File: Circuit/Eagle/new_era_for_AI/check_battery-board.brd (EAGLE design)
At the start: 94 x 70 mm, 32 parts

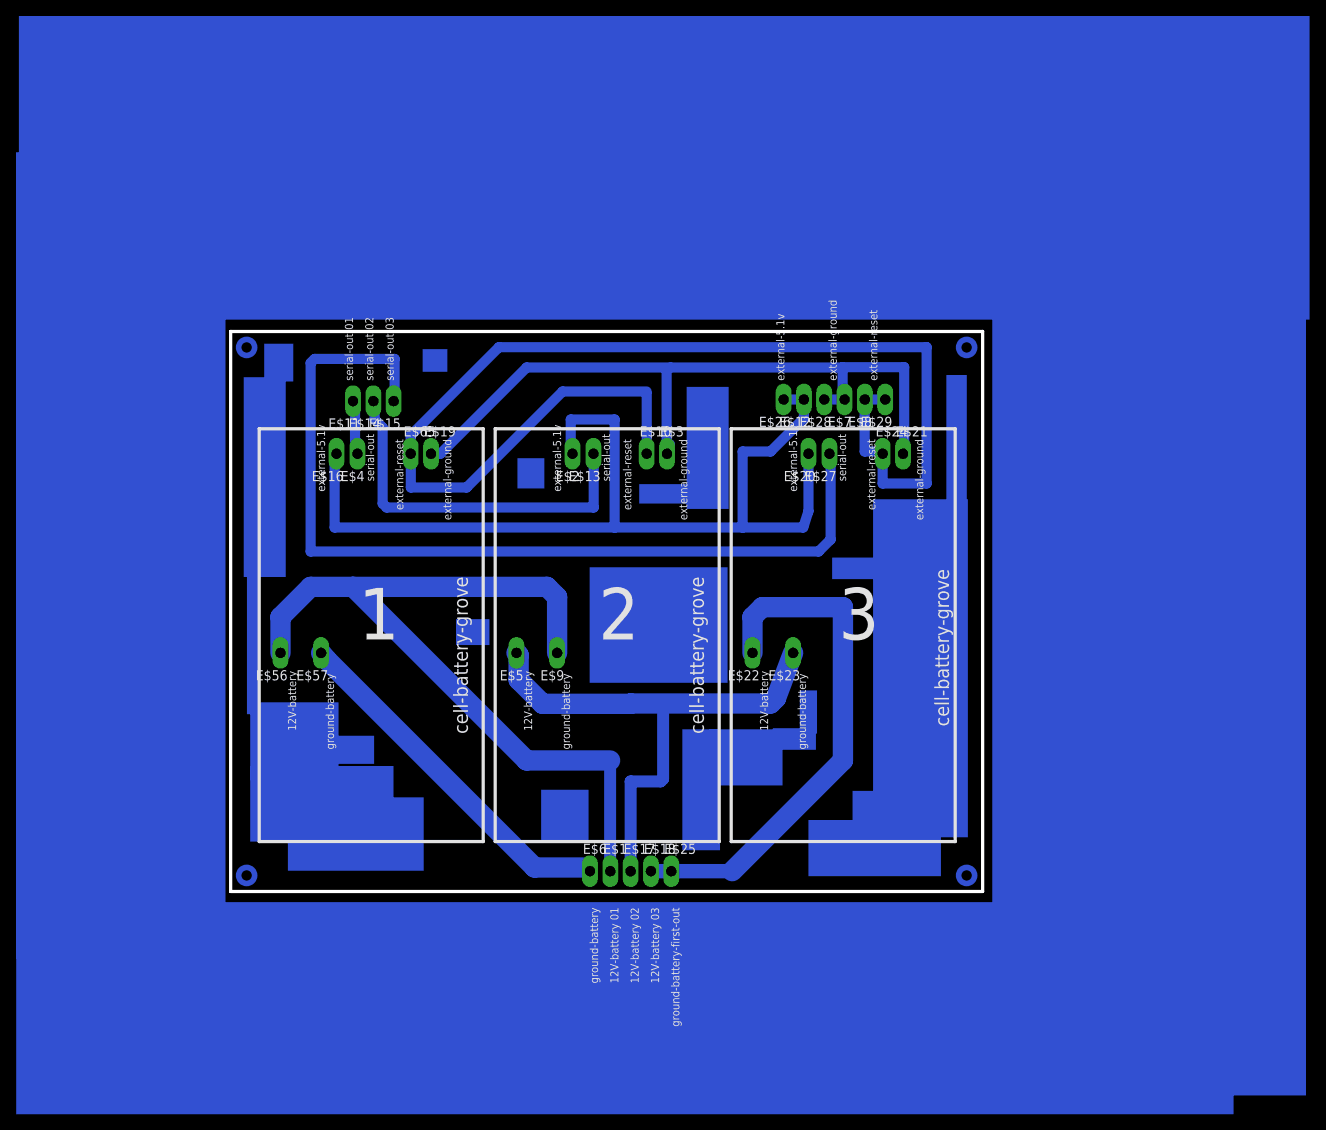
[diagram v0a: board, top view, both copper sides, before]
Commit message: .
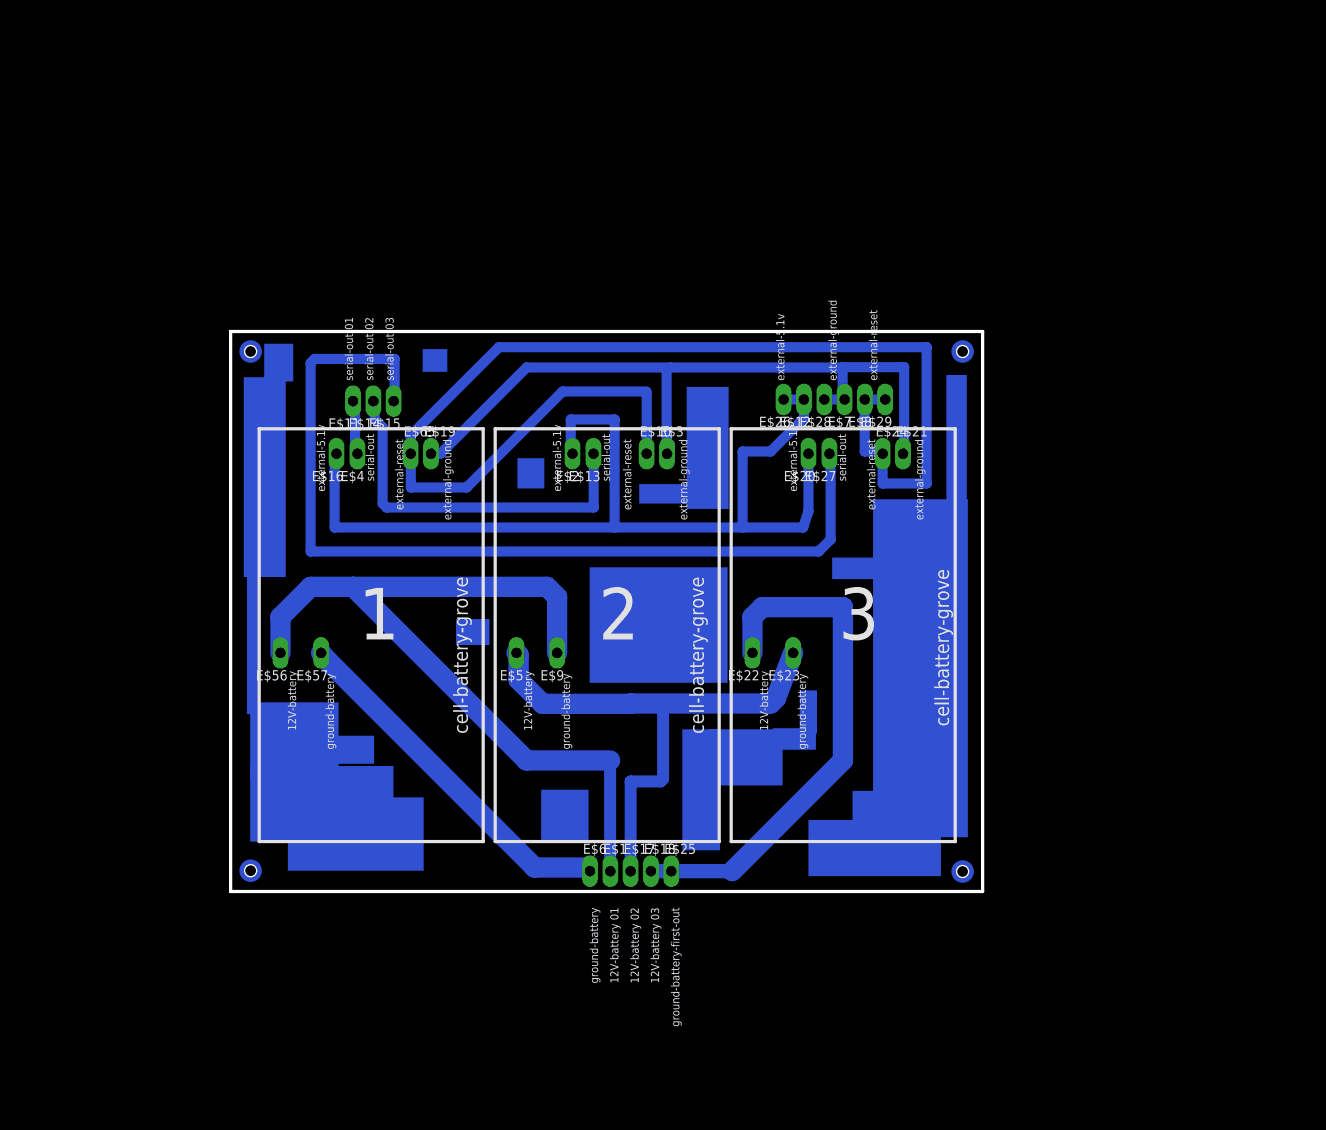
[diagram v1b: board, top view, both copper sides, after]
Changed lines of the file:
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@@
 <setting verticaltext="up"/>
 </settings>
-<grid distance="0.003125" unitdist="mic" unit="mm" style="lines" multiple="1" display="yes" altdistance="0.003125" altunitdist="mic" altunit="mm"/>
+<grid distance="0.5" unitdist="mm" unit="mm" style="lines" multiple="1" display="yes" altdistance="0.003125" altunitdist="mic" altunit="mm"/>
 <layers>
-<layer number="1" name="Top" color="4" fill="1" visible="no" active="yes"/>
+<layer number="1" name="Top" color="4" fill="1" visible="yes" active="yes"/>
 <layer number="2" name="Route2" color="1" fill="3" visible="no" active="no"/>
 <layer number="3" name="Route3" color="4" fill="3" visible="no" active="no"/>
@@
 <layer number="45" name="Holes" color="7" fill="1" visible="yes" active="yes"/>
 <layer number="46" name="Milling" color="3" fill="1" visible="no" active="yes"/>
-<layer number="47" name="Measures" color="7" fill="1" visible="no" active="yes"/>
+<layer number="47" name="Measures" color="7" fill="1" visible="yes" active="yes"/>
 <layer number="48" name="Document" color="7" fill="1" visible="no" active="yes"/>
 <layer number="49" name="Reference" color="7" fill="1" visible="no" active="yes"/>
@@
 </layers>
 <board>
-<fusionsync huburn="a.cGVyc29uYWw6dWUyZDdmOThi" projecturn="a.cGVyc29uYWw6dWUyZDdmOThiIzIwMjAxMTA1MzUwMDc2Njgx" f3durn="urn:adsk.wipprod:dm.lineage:Sfrp7S-jSqKYQXxY8w-WgQ" pcbguid="81441e6f-d9b8-4305-a09b-ce2376f146d5" lastpulledtime="" lastsyncedchangeguid="9a0dcba4-15db-f250-db5e-a71cff48e025" latestrevisionid="" lastsyncedrevisionid="" lastboardhashguid="" lastpushedtime="" linktopcb3d="false"/>
+<fusionsync huburn="a.cGVyc29uYWw6dWUyZDdmOThi" projecturn="a.cGVyc29uYWw6dWUyZDdmOThiIzIwMjAxMTA1MzUwMDc2Njgx" f3durn="urn:adsk.wipprod:dm.lineage:0ixU6gNjSq-owvs7GqFS4g" pcbguid="" lastpulledtime="" lastsyncedchangeguid="9a0dcba4-15db-f250-db5e-a71cff48e025" latestrevisionid="9c5196f6-a430-4b2d-92e1-2361bd45ccda" lastsyncedrevisionid="9c5196f6-a430-4b2d-92e1-2361bd45ccda" lastboardhashguid="3221ca91-becd-a7e8-faa7-446c98a98a6c" lastpushedtime="2024-01-14T22:33:02Z" linktopcb3d="true"/>
 <plain>
 <text x="19.933525" y="53.274865625" size="1.016" layer="21" rot="R90">serial-out</text>
@@
 <text x="48" y="33.5" size="6.4516" layer="21">2</text>
 <text x="78" y="33.5" size="6.4516" layer="21">3</text>
-<wire x1="2" y1="72" x2="96" y2="72" width="0.4064" layer="20"/>
-<wire x1="96" y1="2" x2="2" y2="2" width="0.4064" layer="20"/>
 <dimension x1="2" y1="72" x2="96" y2="72" x3="49" y3="86" textsize="1.778" layer="47"/>
 <dimension x1="2" y1="2" x2="2" y2="72" x3="-8" y3="37" textsize="1.778" layer="47"/>
 <text x="57.08" y="0" size="1.016" layer="21" rot="R270">ground-battery-first-out</text>
-<wire x1="2.001834375" y1="2.008475" x2="2.001834375" y2="72.008475" width="0.4064" layer="20"/>
-<wire x1="96.001834375" y1="72.008475" x2="96.001834375" y2="2.008475" width="0.4064" layer="20"/>
-<circle x="4.001834375" y="70.008475" radius="1" width="0.7" layer="16"/>
-<circle x="94.001834375" y="70.008475" radius="1" width="0.7" layer="16"/>
-<circle x="4.001834375" y="4.008475" radius="1" width="0.7" layer="16"/>
-<circle x="94.001834375" y="4.008475" radius="1" width="0.7" layer="16"/>
 <rectangle x1="9.159853125" y1="4.59029375" x2="26.13251875" y2="13.770884375" layer="16"/>
 <rectangle x1="4.445221875" y1="8.235528125" x2="22.360815625" y2="17.686134375" layer="16"/>
@@
 <rectangle x1="25.997815625" y1="66.964296875" x2="29.096" y2="69.799478125" layer="16"/>
 <rectangle x1="6.196371875" y1="65.74921875" x2="9.833371875" y2="70.474521875" layer="16"/>
-<rectangle x1="-24.8285875" y1="-6.41004375" x2="1.3578125" y2="94.402484375" layer="16"/>
-<rectangle x1="-24.80375625" y1="-25.845303125" x2="127.37064375" y2="0.67130625" layer="16"/>
-<rectangle x1="97.2039125" y1="-23.495728125" x2="136.420665625" y2="98.34640625" layer="16"/>
-<rectangle x1="-24.468571875" y1="73.481246875" x2="136.86758125" y2="111.436884375" layer="16"/>
+<wire x1="2" y1="72" x2="96" y2="72" width="0.4064" layer="20"/>
+<wire x1="96" y1="72" x2="96" y2="2" width="0.4064" layer="20"/>
+<wire x1="96" y1="2" x2="2" y2="2" width="0.4064" layer="20"/>
+<wire x1="2" y1="2" x2="2" y2="72" width="0.4064" layer="20"/>
+<hole x="93.5" y="4.5" drill="1.5"/>
+<hole x="93.5" y="69.5" drill="1.5"/>
+<hole x="4.5" y="69.5" drill="1.5"/>
+<hole x="4.5" y="4.6" drill="1.5"/>
+<circle x="4.5" y="69.5" radius="1" width="0.8128" layer="16"/>
+<circle x="93.5" y="69.5" radius="1" width="0.8128" layer="16"/>
+<circle x="4.5" y="4.6" radius="1" width="0.8128" layer="16"/>
+<circle x="93.5" y="4.5" radius="1" width="0.8128" layer="16"/>
 </plain>
 <attributes>
